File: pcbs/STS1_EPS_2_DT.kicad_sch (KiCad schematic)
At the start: 17 parts, among them Q2 SI7272DP-T1-GE3, Q3 2N7002, U1 4072, U2 LTC6995IDCB-1

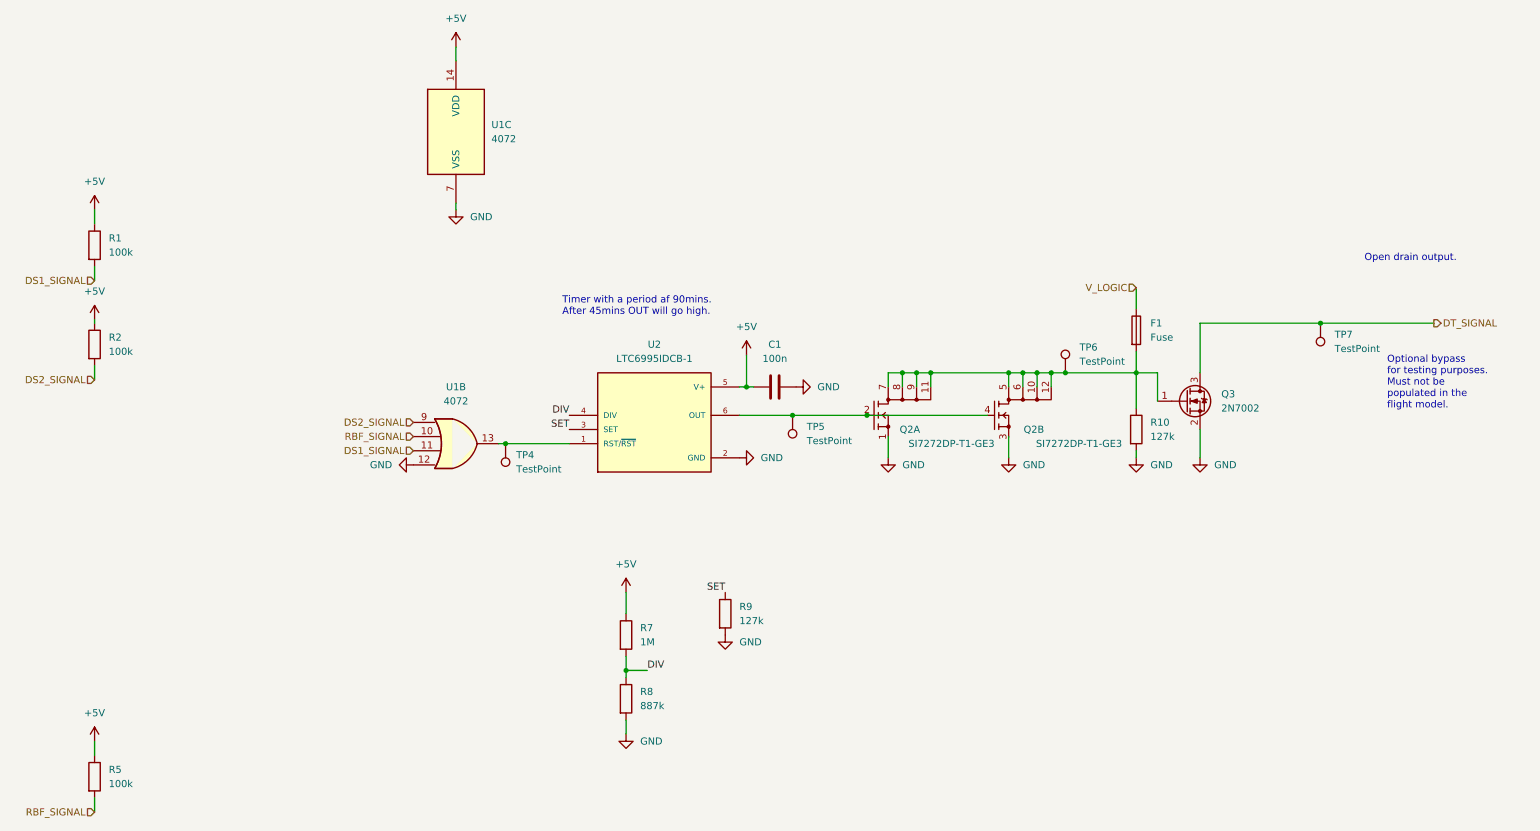
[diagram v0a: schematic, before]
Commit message: Intermediate commit.
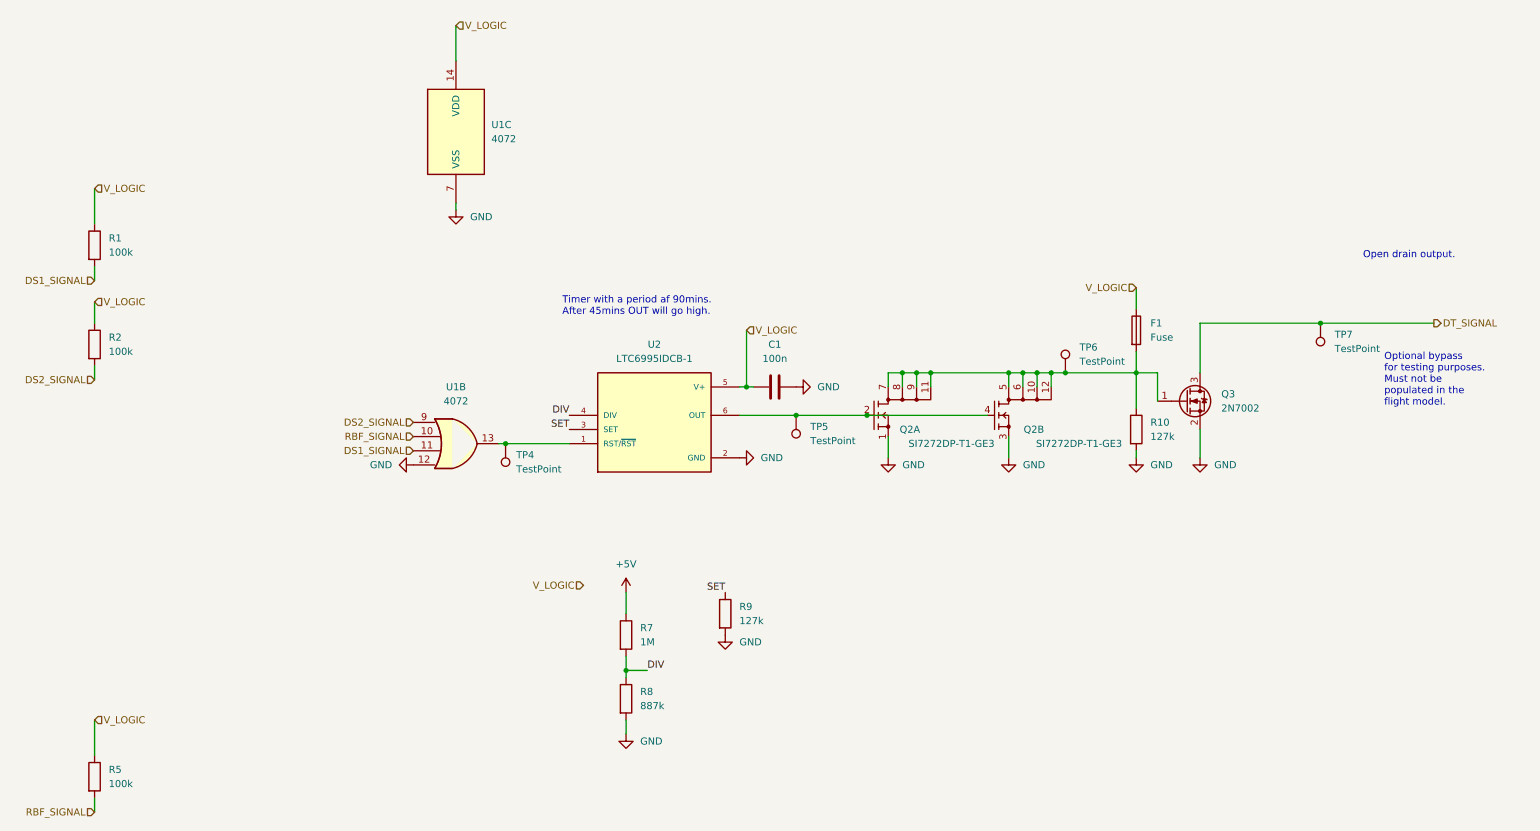
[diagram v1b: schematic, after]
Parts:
- U1: footprint STS_Misc:SOP127P780X200-14N -> Package_SO:SOIC-14_3.9x8.7mm_P1.27mm
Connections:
- net +5V: no longer C1.1, R1.1, R2.1, R5.1, U1.14 (VDD), U2.5 (V+)
- net V_LOGIC: now also C1.1, R1.1, R2.1, R5.1, U1.14 (VDD), U2.5 (V+)
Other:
- moved on the sheet: TP5
